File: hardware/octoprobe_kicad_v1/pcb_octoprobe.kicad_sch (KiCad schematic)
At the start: 12 parts, among them J101 Conn_01x20, J102 Conn_01x20, J103 Conn_01x20

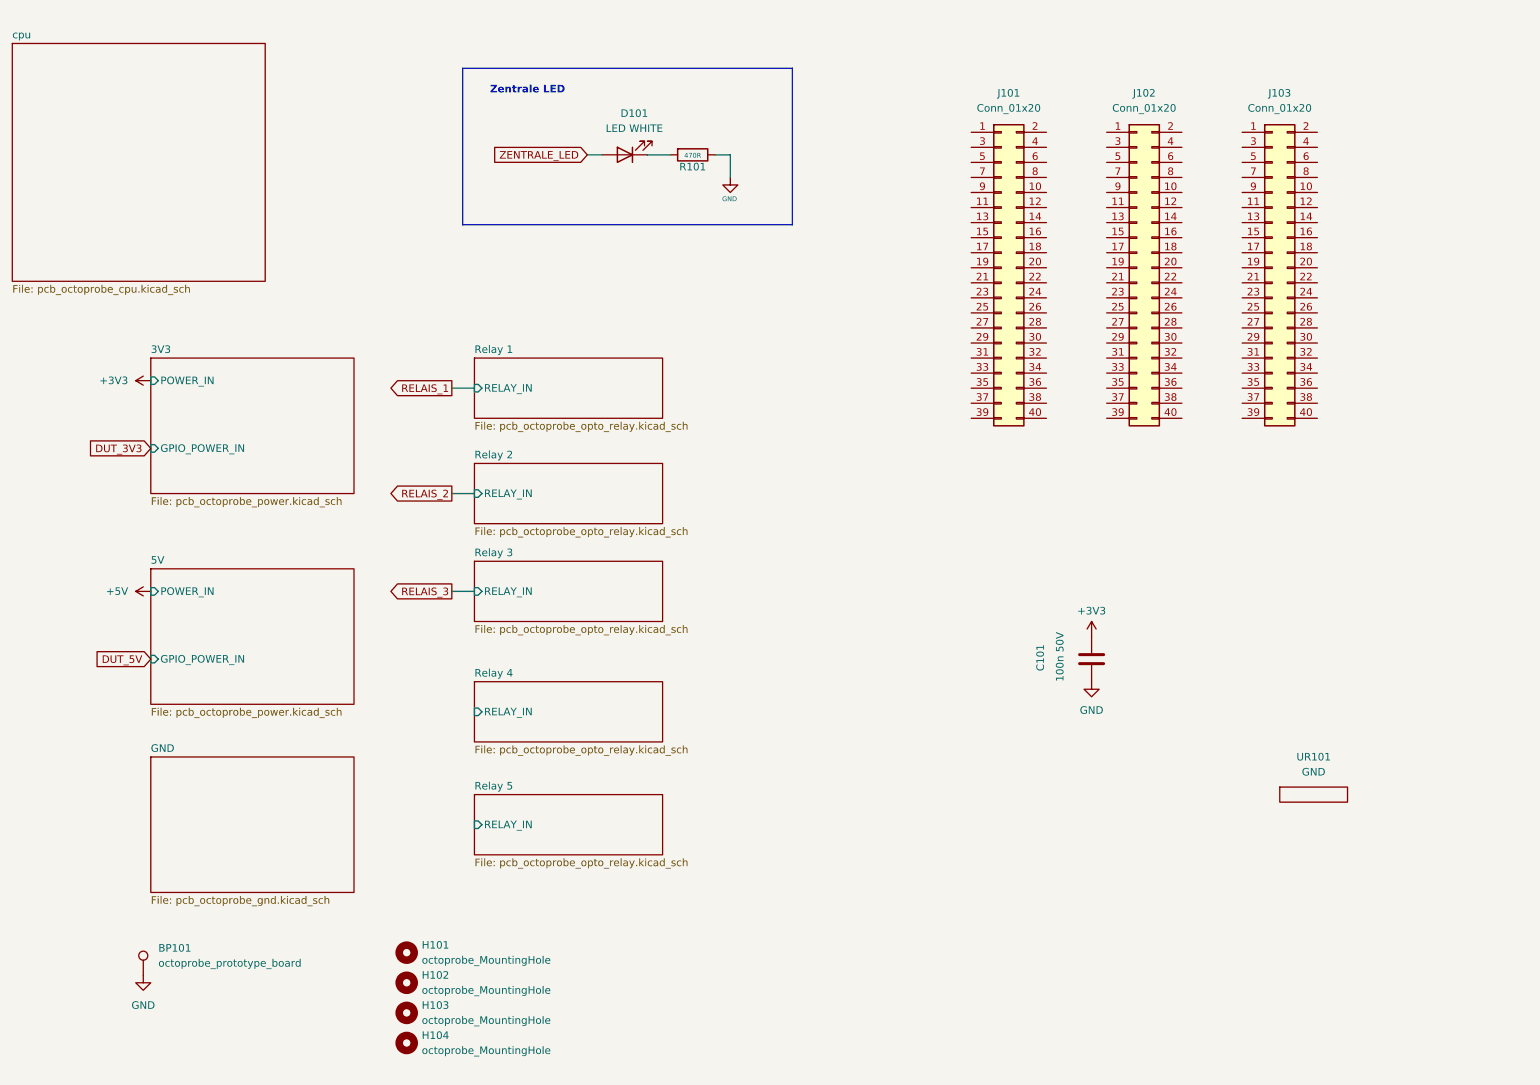
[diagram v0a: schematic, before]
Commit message: Relay
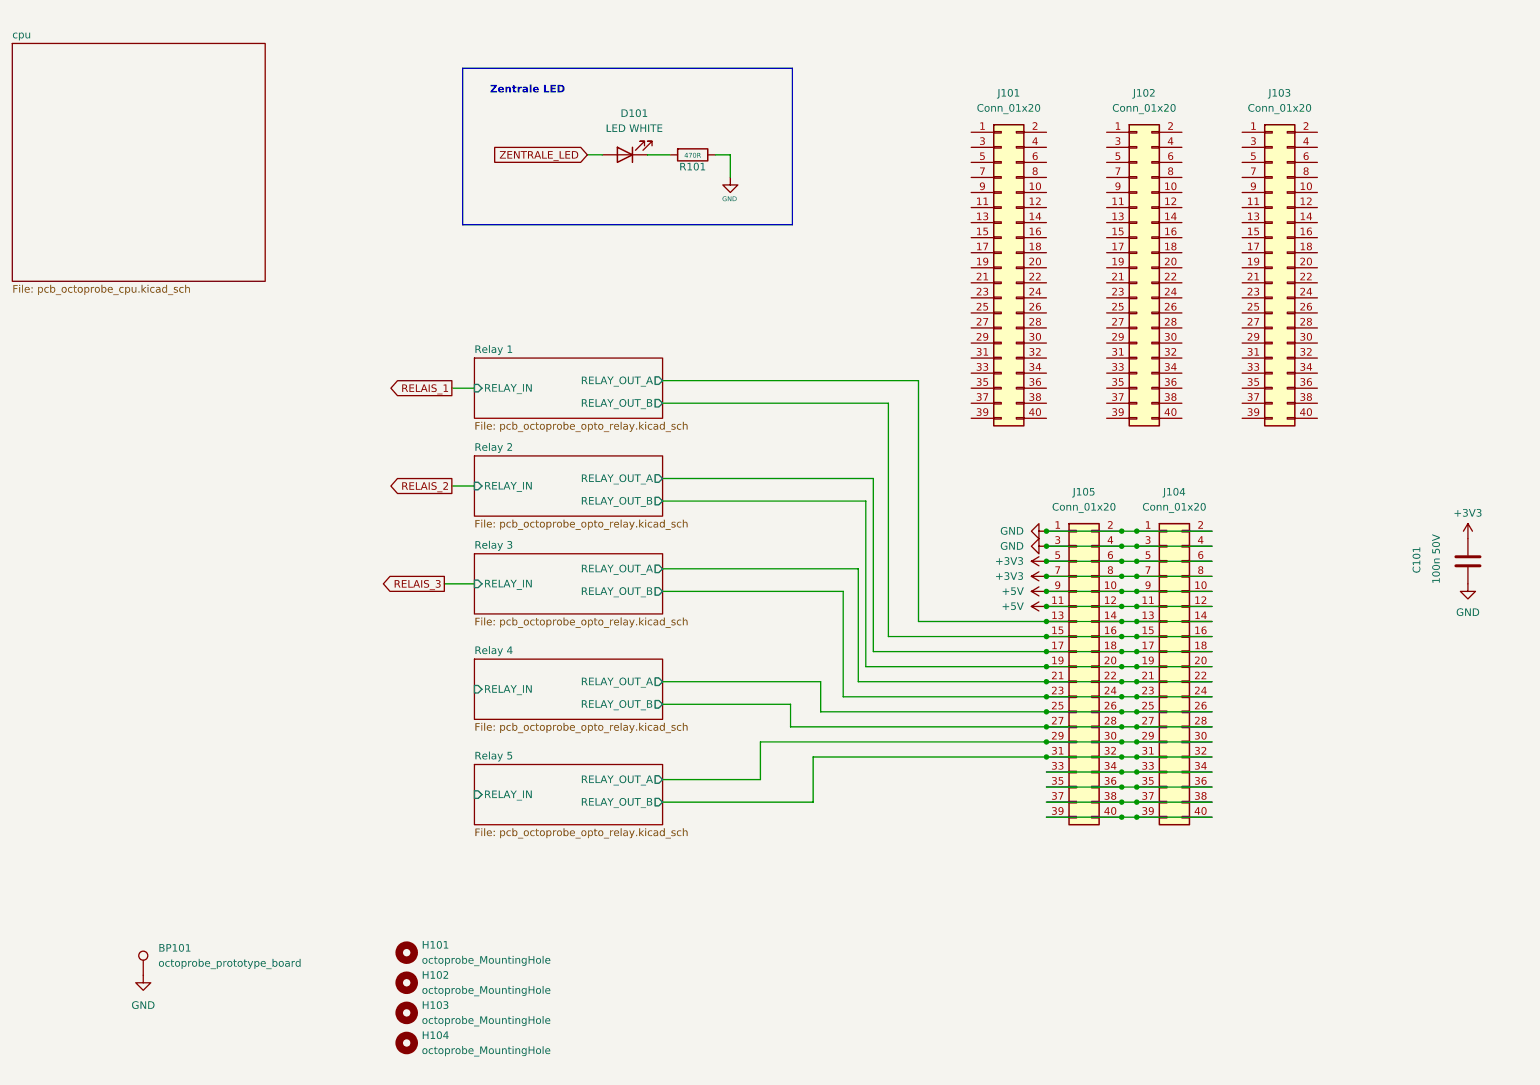
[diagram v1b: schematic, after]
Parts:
- removed UR101: GND, 00_project_library:opctoprobe_relay, symbol 00_project_library:opctoprobe_relay
- added J104: Conn_01x20, 00_project_library:PinSocket_2x20_P2.54mm_Vertical-mirrored, symbol Connector_Generic:Conn_02x20_Odd_Even
- added J105: Conn_01x20, 00_project_library:PinSocket_2x20_P2.54mm_Vertical-mirrored-bare, symbol Connector_Generic:Conn_02x20_Odd_Even
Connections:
- net +3V3: now also J104.5 (Pin_5), J104.6 (Pin_6), J104.7 (Pin_7), J104.8 (Pin_8), J105.5 (Pin_5), J105.6 (Pin_6), J105.7 (Pin_7), J105.8 (Pin_8)
- net +5V: now also J104.10 (Pin_10), J104.11 (Pin_11), J104.12 (Pin_12), J104.9 (Pin_9), J105.10 (Pin_10), J105.11 (Pin_11), J105.12 (Pin_12), J105.9 (Pin_9)
- net GND: now also J104.1 (Pin_1), J104.2 (Pin_2), J104.3 (Pin_3), J104.4 (Pin_4), J105.1 (Pin_1), J105.2 (Pin_2), J105.3 (Pin_3), J105.4 (Pin_4)
- new net: J104.33 (Pin_33), J104.34 (Pin_34), J105.33 (Pin_33), J105.34 (Pin_34)
- new net: J104.35 (Pin_35), J104.36 (Pin_36), J105.35 (Pin_35), J105.36 (Pin_36)
- new net: J104.37 (Pin_37), J104.38 (Pin_38), J105.37 (Pin_37), J105.38 (Pin_38)
- new net: J104.39 (Pin_39), J104.40 (Pin_40), J105.39 (Pin_39), J105.40 (Pin_40)
- new net Relay 1/RELAY_OUT_A: J104.13 (Pin_13), J104.14 (Pin_14), J105.13 (Pin_13), J105.14 (Pin_14)
- new net Relay 1/RELAY_OUT_B: J104.15 (Pin_15), J104.16 (Pin_16), J105.15 (Pin_15), J105.16 (Pin_16)
- new net Relay 2/RELAY_OUT_A: J104.17 (Pin_17), J104.18 (Pin_18), J105.17 (Pin_17), J105.18 (Pin_18)
- new net Relay 2/RELAY_OUT_B: J104.19 (Pin_19), J104.20 (Pin_20), J105.19 (Pin_19), J105.20 (Pin_20)
- new net Relay 3/RELAY_OUT_A: J104.21 (Pin_21), J104.22 (Pin_22), J105.21 (Pin_21), J105.22 (Pin_22)
- new net Relay 3/RELAY_OUT_B: J104.23 (Pin_23), J104.24 (Pin_24), J105.23 (Pin_23), J105.24 (Pin_24)
- new net Relay 4/RELAY_OUT_A: J104.25 (Pin_25), J104.26 (Pin_26), J105.25 (Pin_25), J105.26 (Pin_26)
- new net Relay 4/RELAY_OUT_B: J104.27 (Pin_27), J104.28 (Pin_28), J105.27 (Pin_27), J105.28 (Pin_28)
- new net Relay 5/RELAY_OUT_A: J104.29 (Pin_29), J104.30 (Pin_30), J105.29 (Pin_29), J105.30 (Pin_30)
- new net Relay 5/RELAY_OUT_B: J104.31 (Pin_31), J104.32 (Pin_32), J105.31 (Pin_31), J105.32 (Pin_32)
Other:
- removed sheet 3V3
- removed sheet 5V
- removed sheet GND
- sheet Relay 1 ports: added RELAY_OUT_A, RELAY_OUT_B; removed none
- sheet Relay 2 ports: added RELAY_OUT_A, RELAY_OUT_B; removed none
- sheet Relay 3 ports: added RELAY_OUT_A, RELAY_OUT_B; removed none
- sheet Relay 4 ports: added RELAY_OUT_A, RELAY_OUT_B; removed none
- sheet Relay 5 ports: added RELAY_OUT_A, RELAY_OUT_B; removed none
- moved on the sheet: C101

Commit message: Improve PCB
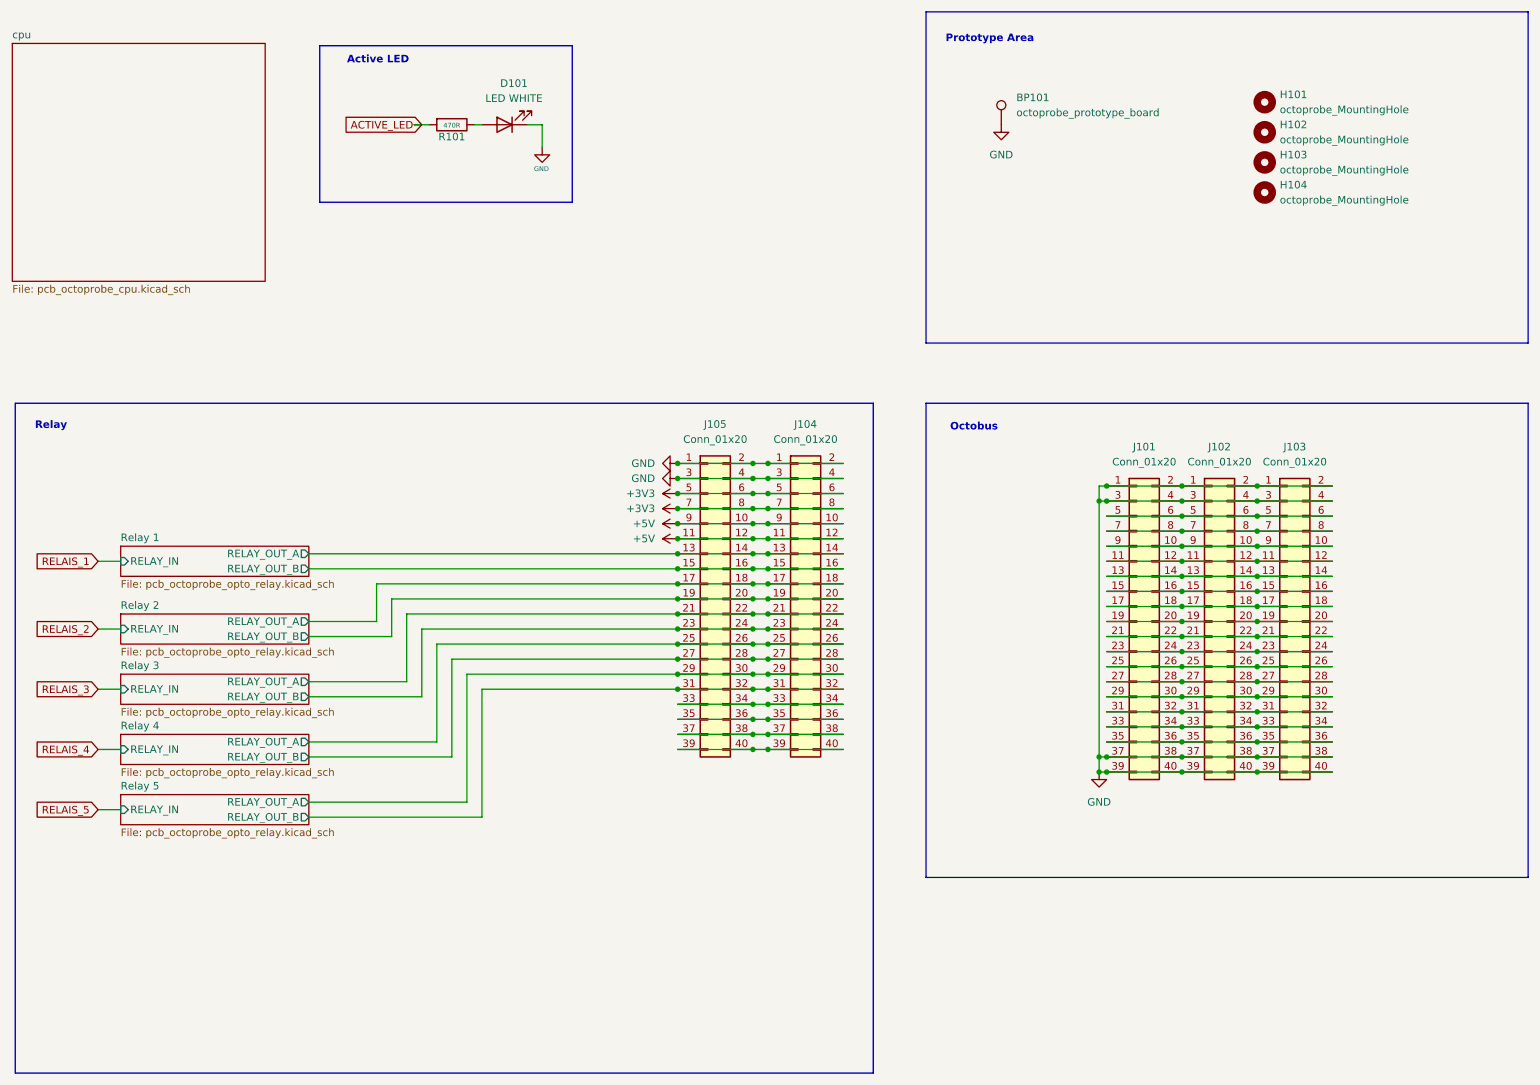
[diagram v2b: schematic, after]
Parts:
- removed C101: 100n 50V, Diode_SMD:D_0805_2012Metric, symbol Device:C
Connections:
- net GND: now also D101.1 (K), J101.1 (Pin_1), J101.2 (Pin_2), J101.3 (Pin_3), J101.37 (Pin_37), J101.38 (Pin_38), J101.39 (Pin_39), J101.4 (Pin_4), J101.40 (Pin_40), J102.1 (Pin_1), J102.2 (Pin_2), J102.3 (Pin_3), J102.37 (Pin_37), J102.38 (Pin_38), J102.39 (Pin_39), J102.4 (Pin_4), J102.40 (Pin_40), J103.1 (Pin_1), J103.2 (Pin_2), J103.3 (Pin_3), J103.37 (Pin_37), J103.38 (Pin_38), J103.39 (Pin_39), J103.4 (Pin_4), J103.40 (Pin_40); no longer R101.1
- net at J102.10 (Pin_10): now also J101.10 (Pin_10), J101.9 (Pin_9), J102.9 (Pin_9), J103.10 (Pin_10), J103.9 (Pin_9)
- net at J102.11 (Pin_11): now also J101.11 (Pin_11), J101.12 (Pin_12), J102.12 (Pin_12), J103.11 (Pin_11), J103.12 (Pin_12)
- net at J102.13 (Pin_13): now also J101.13 (Pin_13), J101.14 (Pin_14), J102.14 (Pin_14), J103.13 (Pin_13), J103.14 (Pin_14)
- net at J102.15 (Pin_15): now also J101.15 (Pin_15), J101.16 (Pin_16), J102.16 (Pin_16), J103.15 (Pin_15), J103.16 (Pin_16)
- net at J102.17 (Pin_17): now also J101.17 (Pin_17), J101.18 (Pin_18), J102.18 (Pin_18), J103.17 (Pin_17), J103.18 (Pin_18)
- net at J102.19 (Pin_19): now also J101.19 (Pin_19), J101.20 (Pin_20), J102.20 (Pin_20), J103.19 (Pin_19), J103.20 (Pin_20)
- net at J102.21 (Pin_21): now also J101.21 (Pin_21), J101.22 (Pin_22), J102.22 (Pin_22), J103.21 (Pin_21), J103.22 (Pin_22)
- net at J102.23 (Pin_23): now also J101.23 (Pin_23), J101.24 (Pin_24), J102.24 (Pin_24), J103.23 (Pin_23), J103.24 (Pin_24)
- net at J102.25 (Pin_25): now also J101.25 (Pin_25), J101.26 (Pin_26), J102.26 (Pin_26), J103.25 (Pin_25), J103.26 (Pin_26)
- net at J102.27 (Pin_27): now also J101.27 (Pin_27), J101.28 (Pin_28), J102.28 (Pin_28), J103.27 (Pin_27), J103.28 (Pin_28)
- net at J102.29 (Pin_29): now also J101.29 (Pin_29), J101.30 (Pin_30), J102.30 (Pin_30), J103.29 (Pin_29), J103.30 (Pin_30)
- net at J102.31 (Pin_31): now also J101.31 (Pin_31), J101.32 (Pin_32), J102.32 (Pin_32), J103.31 (Pin_31), J103.32 (Pin_32)
- net at J102.33 (Pin_33): now also J101.33 (Pin_33), J101.34 (Pin_34), J102.34 (Pin_34), J103.33 (Pin_33), J103.34 (Pin_34)
- net at J102.35 (Pin_35): now also J101.35 (Pin_35), J101.36 (Pin_36), J102.36 (Pin_36), J103.35 (Pin_35), J103.36 (Pin_36)
- net at J102.5 (Pin_5): now also J101.5 (Pin_5), J101.6 (Pin_6), J102.6 (Pin_6), J103.5 (Pin_5), J103.6 (Pin_6)
- net at J102.7 (Pin_7): now also J101.7 (Pin_7), J101.8 (Pin_8), J102.8 (Pin_8), J103.7 (Pin_7), J103.8 (Pin_8)
- net ACTIVE_LED: now reaches R101.2
- net ACTIVE_LED: no longer D101.1 (K)
- net ZENTRALE_LED: no longer names the net of D101.2 (A)
- net ZENTRALE_LED: now also R101.1
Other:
- note added: "Active LED"
- note added: "Octobus"
- note added: "Prototype Area"
- note added: "Relay"
- note removed: "Zentrale LED"
- moved on the sheet: BP101, D101, H101, H102, H103, H104, J101, J102, J103, J104, J105, R101
